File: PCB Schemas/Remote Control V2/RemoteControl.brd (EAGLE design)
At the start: 62.5 x 60.3 mm, 23 parts, among them IC1 ATMEGA328-PU, Q1 16MHz

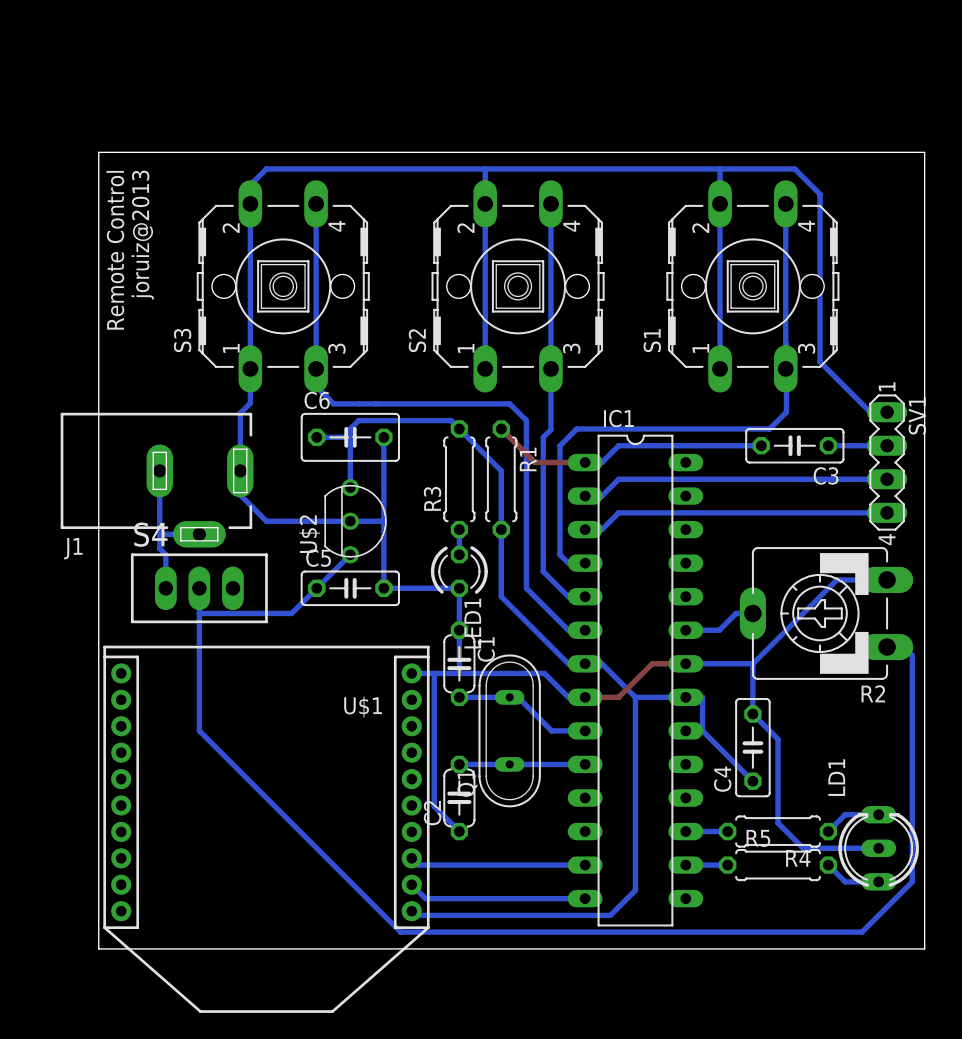
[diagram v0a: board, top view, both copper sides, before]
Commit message: Finalized V1 and V2 of remote control
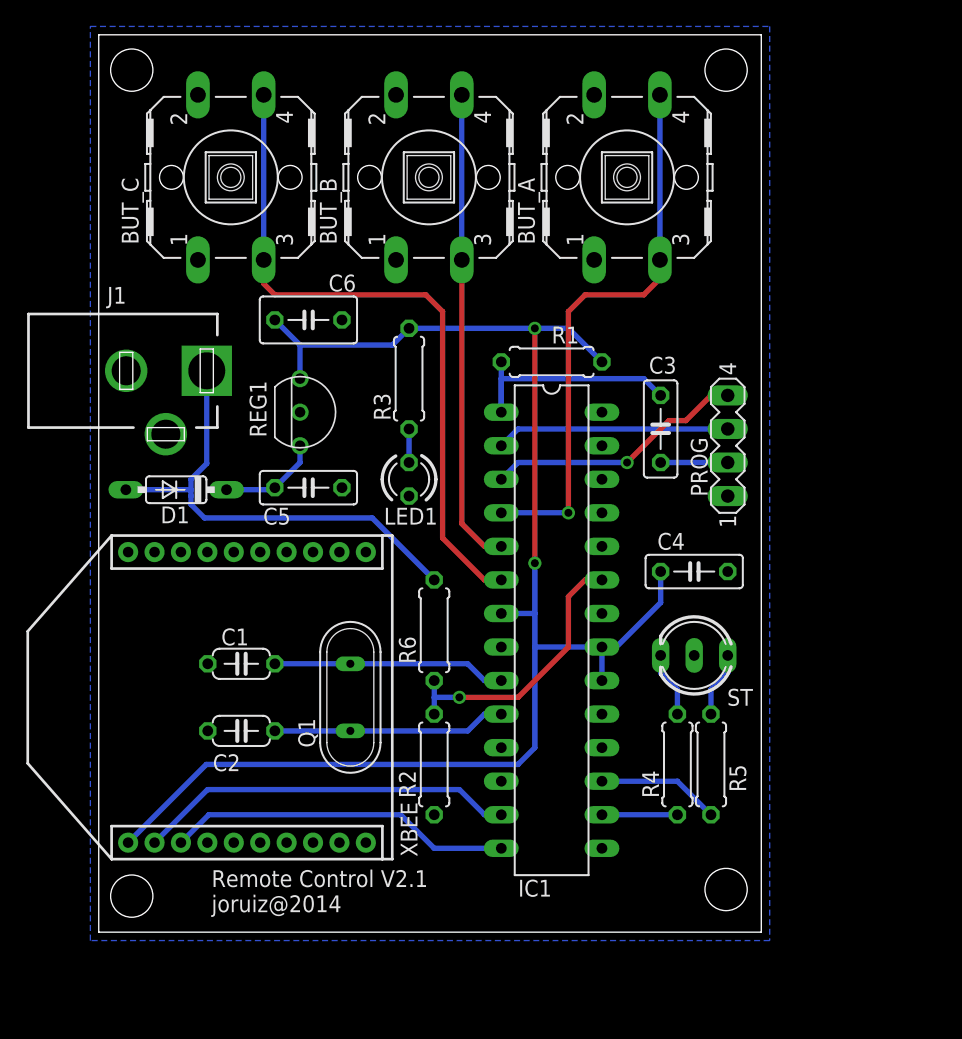
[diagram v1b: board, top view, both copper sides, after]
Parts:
- removed LD1: (no value), led:DUOLED-C-5MM
- removed S1, S2, S3: (no value), switch-omron:B3F-40XX
- removed S4: TL39PO, switch:TL3XPO
- removed SV1: (no value), con-lstb:MA04-1
- removed U$1: XBEE-1B1, Xbee:XBEE-1
- removed U$2: LE33, Regulator:TO-92
- added BUT_A, BUT_B, BUT_C: (no value), switch-omron:B3F-40XX
- added D1: (no value), diode:DO35-7
- added PROG: (no value), con-lstb:MA04-1
- added R6: 330k, resistor:0207/7
- added REG1: LE33, Regulator:TO-92
- added ST: (no value), led:DUOLED-C-5MM
- added XBEE: XBEE-1B1, Xbee:XBEE-1
- J1: device con-jack:DCJ0303 -> Connectors:DCJ0303
- R2: value (none) -> 100k; device pot:CA9V -> resistor:0207/7
- R3: value 220 -> 330
- moved R2 31.4 mm to (25.4, 14.0)
- moved C2 17.3 mm to (10.8, 16.5), turned to 0 degrees
- moved C1 16.5 mm to (10.8, 21.6), turned to 0 degrees
- moved C4 14.1 mm to (45.1, 28.6), turned to 0 degrees
- moved Q1 12.3 mm to (19.1, 19.1)
- moved C3 10.2 mm to (42.5, 39.4), turned to 90 degrees
- moved R1 9.67 mm to (34.3, 44.5), turned to 0 degrees
- moved C6 9.44 mm to (15.9, 47.6)
- moved R4 9.16 mm to (43.8, 14.0), turned to 270 degrees
- moved R5 9.16 mm to (46.4, 14.0), turned to 90 degrees
- moved R3 8.52 mm to (23.5, 43.2)
- moved C5 8.25 mm to (15.9, 34.9)
- moved J1 7.99 mm to (5.08, 43.8)
- moved LED1 7.96 mm to (23.5, 35.6)
- moved IC1 7.41 mm to (34.3, 24.1)
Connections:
- removed net BLUE_BUTTON: IC1.6, S3.3, S3.4
- removed net GREEN_BUTTON: IC1.5, S2.3, S2.4
- removed net N$9: IC1.23, R2.S
- removed net RED_BUTTON: IC1.4, S1.3, S1.4
- new net BAT: IC1.23, R2.2, R6.1
- new net BUTTON_A: BUT_A.3, BUT_A.4, IC1.4
- new net BUTTON_B: BUT_B.3, BUT_B.4, IC1.5
- new net BUTTON_C: BUT_C.3, BUT_C.4, IC1.6
- net GND: now also BUT_A.1, BUT_A.2, BUT_B.1, BUT_B.2, BUT_C.1, BUT_C.2, J1.2, J1.3, PROG.1, R2.1, REG1.2, ST.C, XBEE.10; no longer J1.1, LD1.C, R2.E, S1.1, S1.2, S2.1, S2.2, S3.1, S3.2, SV1.1, U$1.10, U$2.2
- net GREEN_LED: now also IC1.17; no longer IC1.16
- net N$11: now also ST.AR; no longer LD1.AR
- net N$12: now also ST.AX; no longer LD1.AX
- net N$3: now also C5.1, D1.C, REG1.1; no longer J1.2, J1.3, S4.1
- net N$6: now also PROG.2; no longer SV1.2
- net RED_LED: now also IC1.16; no longer IC1.17
- net RX: now also PROG.3; no longer SV1.3
- net TX: now also PROG.4; no longer SV1.4
- net VCC: now also REG1.3, XBEE.1; no longer U$1.1, U$2.3
- net VIN: now also D1.A, J1.1, R6.2; no longer C5.1, R2.A, S4.2, U$2.1
- net XBEE_RX: now also IC1.13, XBEE.2; no longer IC1.14, U$1.2
- net XBEE_TX: now also IC1.14, XBEE.3; no longer IC1.13, U$1.3
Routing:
- net GND: track 227.6 -> 0.00 mm
- net VIN: track 105.2 -> 36.3 mm
- net BUTTON_C: track 0.00 -> 51.6 mm
- net BLUE_BUTTON: track 49.3 -> 0.00 mm
- net RED_BUTTON: track 48.1 -> 0.00 mm
- net BUTTON_A: track 0.00 -> 42.2 mm, vias 0 -> 1
- net BUTTON_B: track 0.00 -> 36.2 mm
- net GREEN_BUTTON: track 32.0 -> 0.00 mm
- net VCC: track 89.8 -> 113.5 mm, vias 0 -> 2
- net BAT: track 0.00 -> 21.2 mm, vias 0 -> 1
- net XBEE_RX: track 13.6 -> 28.7 mm
- net XBEE_TX: track 13.3 -> 26.2 mm
- net N$2: track 9.52 -> 17.7 mm
- net N$1: track 10.6 -> 17.7 mm
- net GREEN_LED: track 3.17 -> 9.31 mm
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- added copper zone on layer 16, net GND
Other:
- board size 62.5 x 60.3 mm -> 50.2 x 67.9 mm
- board text added: "Remote Control V2.1 joruiz@2014"
- board text removed: "Remote Control joruiz@2013"
